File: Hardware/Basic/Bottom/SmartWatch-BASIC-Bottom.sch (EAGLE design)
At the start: 32 parts

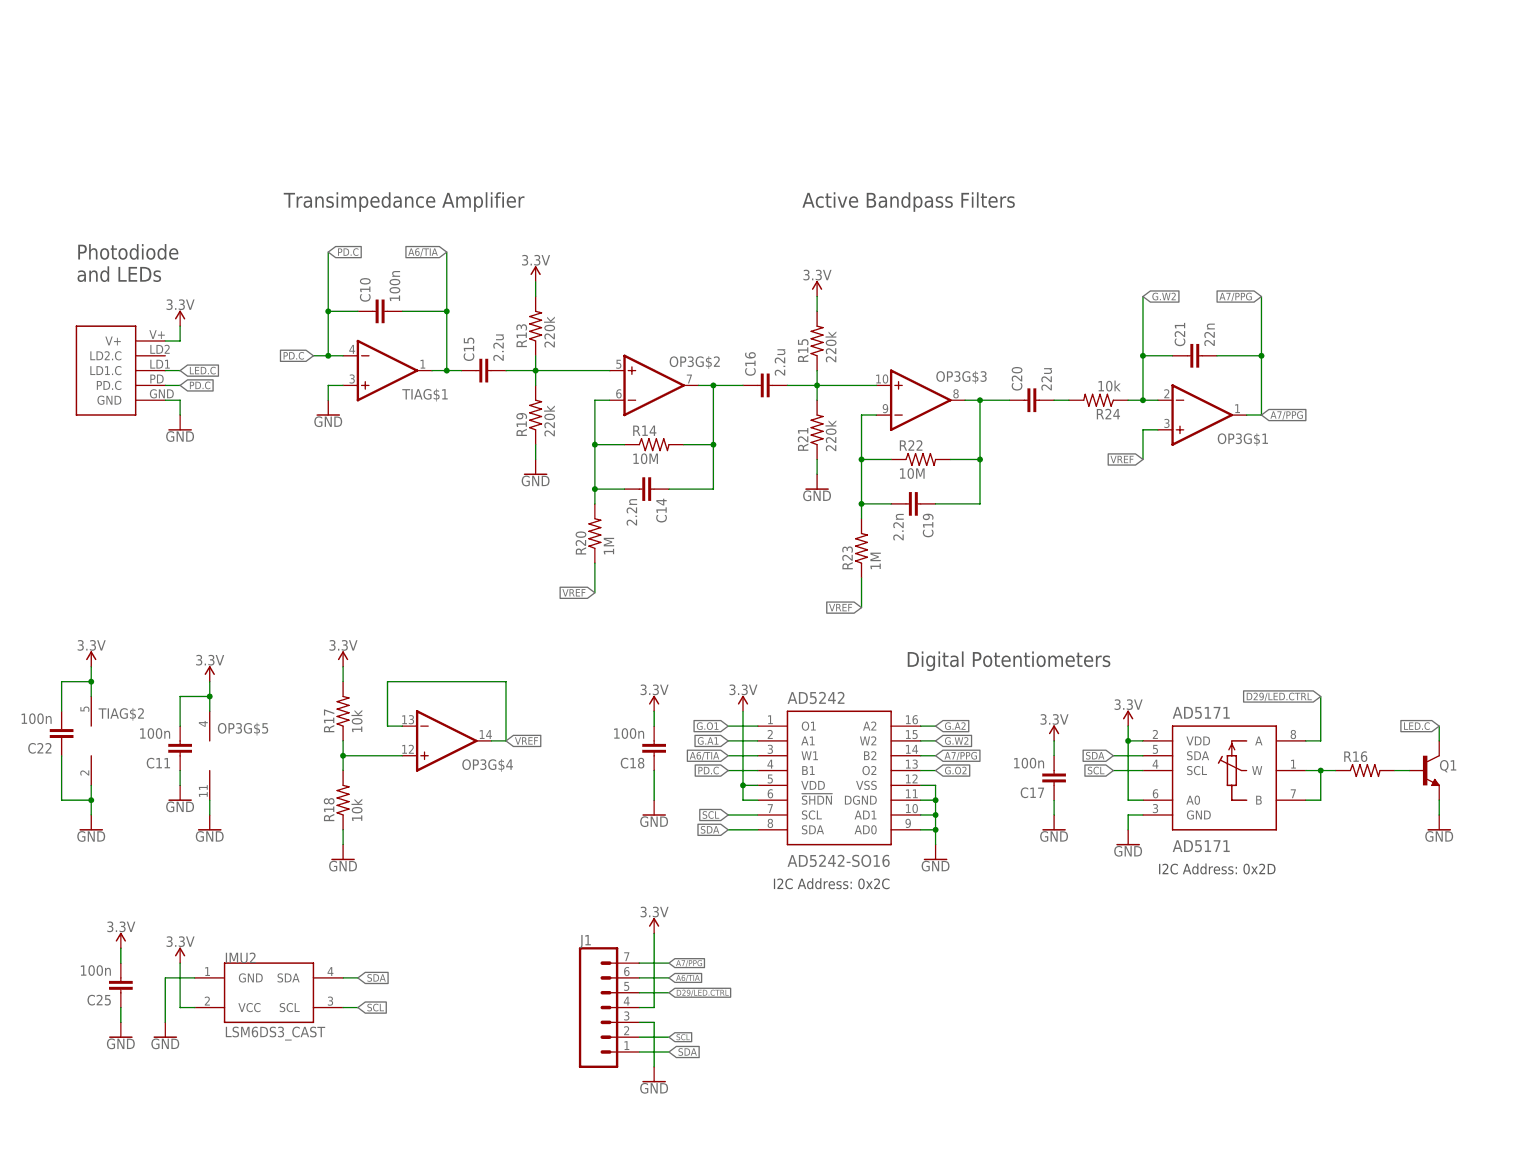
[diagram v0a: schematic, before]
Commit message: Take5
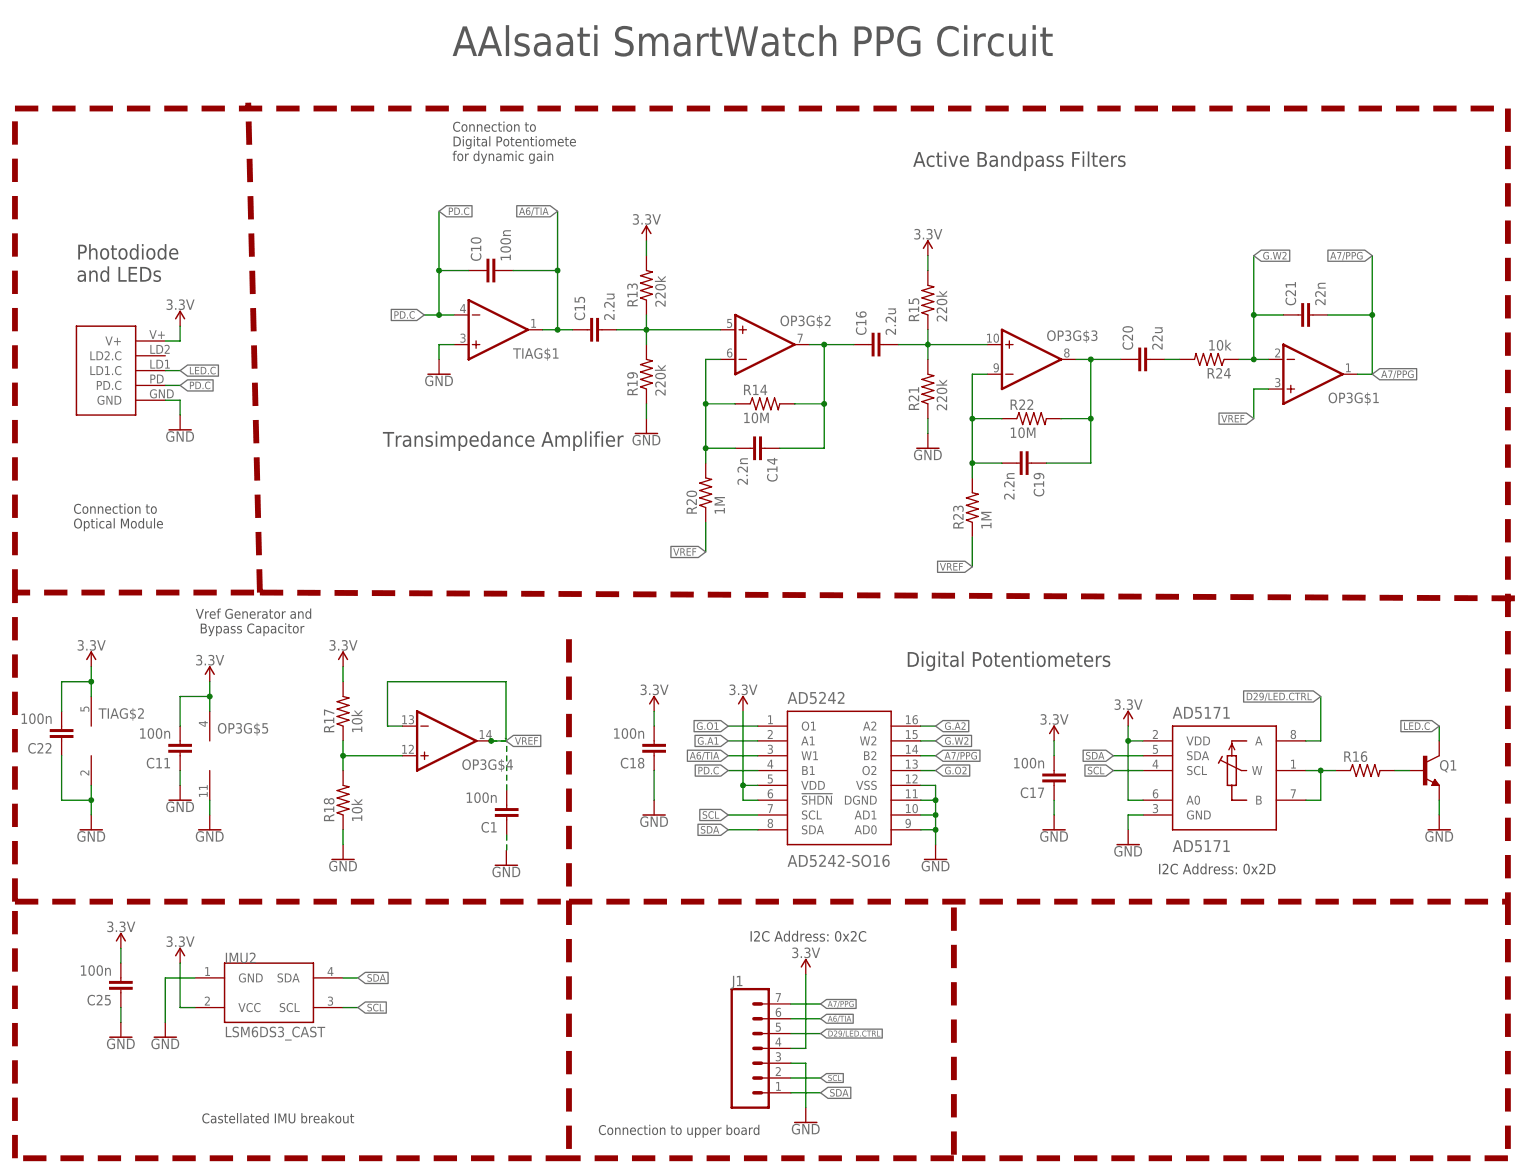
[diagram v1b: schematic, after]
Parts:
- added C1: 100n, LinnesLab-Passives:CAPACITOR0603
- added LOGO1: REVISION.A, LinnesLab-Logos:REVISION.A
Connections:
- net GND: now also C1.1
- net VREF: now also C1.2
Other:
- note added: "AAlsaati SmartWatch PPG Circuit"
- note added: "Castellated IMU breakout"
- note added: "Connection to Digital Potentiomete for dynamic gain"
- note added: "Connection to Optical Module"
- note added: "Connection to upper board"
- note added: "Vref Generator and Bypass Capacitor"
- moved on the sheet: C10, C14, C15, C16, C19, C20, C21, J1, OP3G$1, OP3G$2, OP3G$3, R13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
